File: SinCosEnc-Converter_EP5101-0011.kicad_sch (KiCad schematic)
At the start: 34 parts, among them J1 Conn_01x05_Pin, U2 AM26LS31CDR, U3 AP22652AW6-7, X2 D-SUB-DR-15PCG-AB

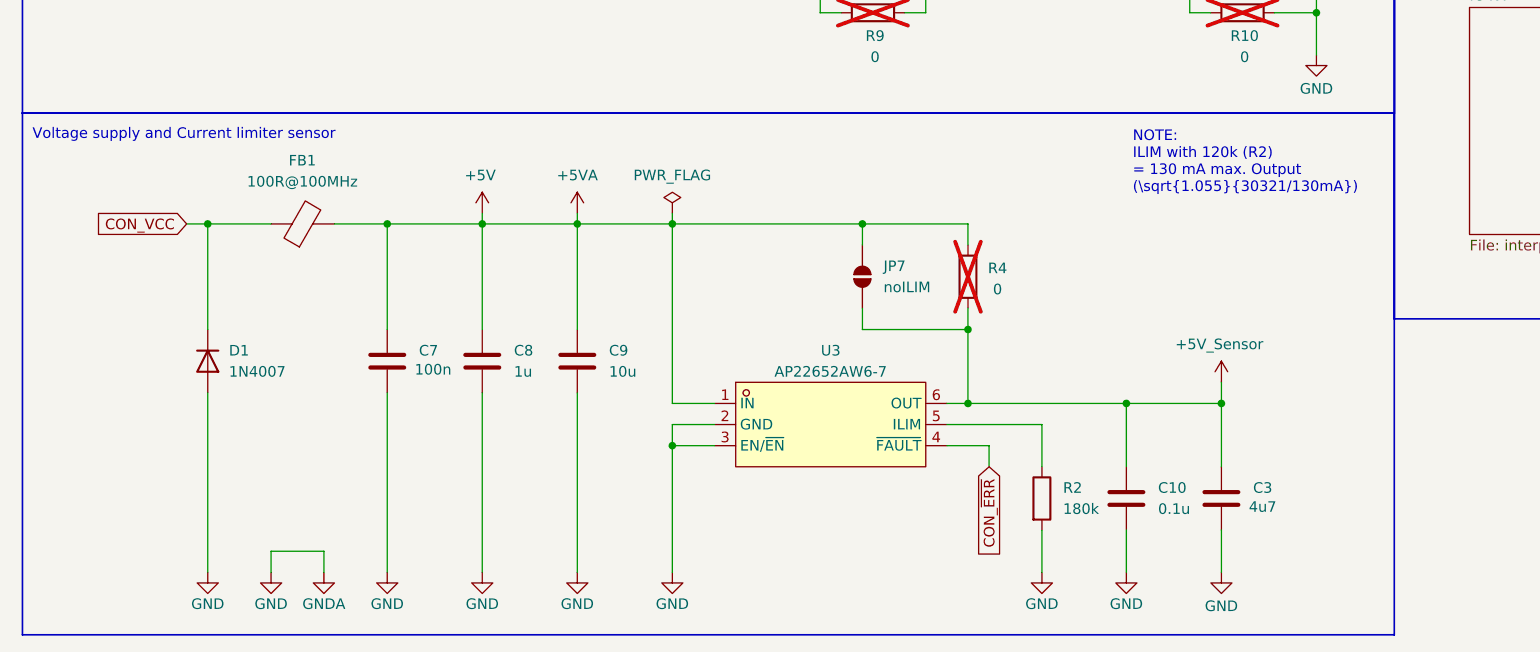
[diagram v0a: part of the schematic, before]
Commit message: v0.9.2 finished, board routed
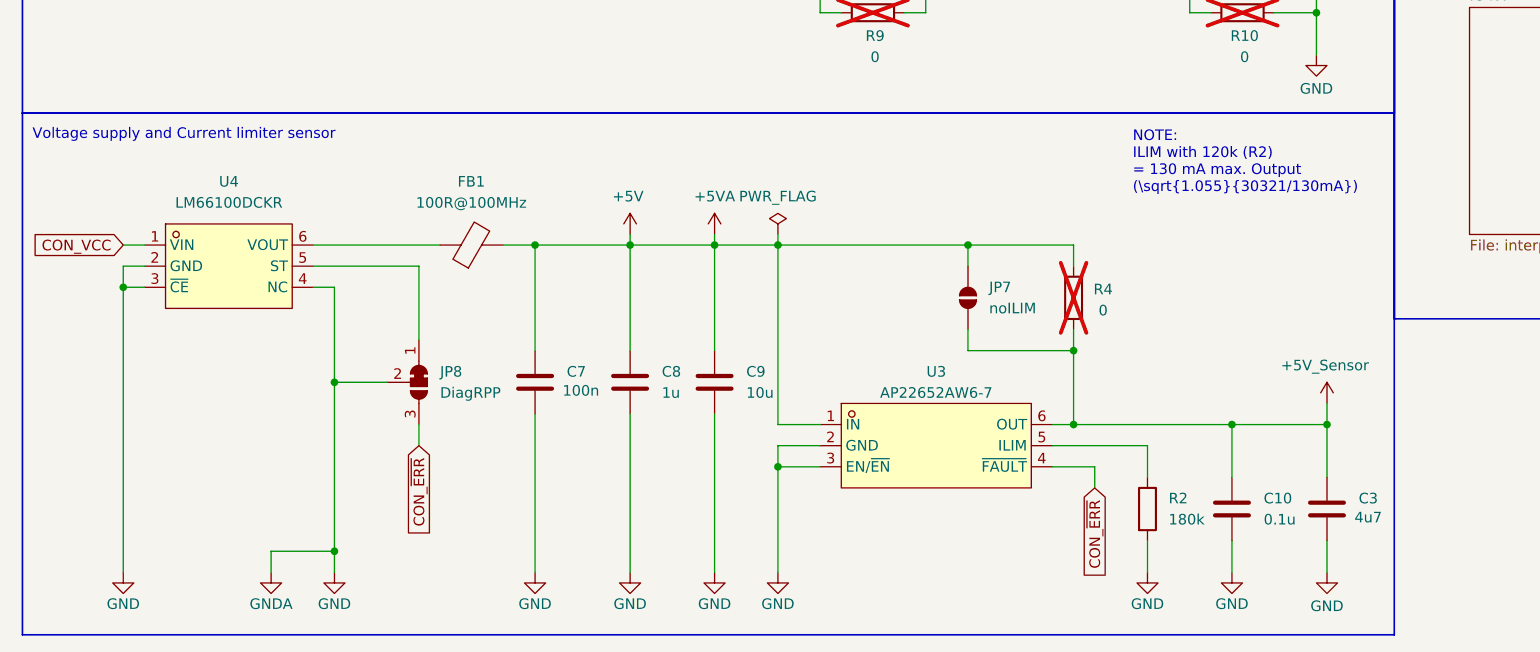
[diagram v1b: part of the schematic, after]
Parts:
- removed D1: 1N4007, Diode_SMD:D_SMA, symbol Diode:1N4007
- added JP8: DiagRPP, Jumper:SolderJumper-3_P1.3mm_Bridged12_RoundedPad1.0x1.5mm, symbol Jumper:SolderJumper_3_Bridged12
- added U4: LM66100DCKR, easyeda2kicad:SC-70-6_L2.0-W1.3-P0.65-LS2.1-BL, symbol easyeda2kicad:LM66100DCKR
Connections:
- net CON_VCC: now also U4.1 (VIN); no longer FB1.1
- net CON_~{ERR}: now also JP8.3 (B)
- net GND: now also JP8.2 (C), U4.2 (GND), U4.3 (~{CE}), U4.4 (NC)
- new net: FB1.1, U4.6 (VOUT)
- new net: JP8.1 (A), U4.5 (ST)
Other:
- moved on the sheet: C10, C3, C7, C8, C9, FB1, JP7, R2, R4, U3
